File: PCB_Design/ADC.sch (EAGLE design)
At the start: 15 parts, among them J1-0 AD_CH0- GND option, J1-1 AD_CH1- GND option, J1-2 AD_CH2- GND option, J1-3 AD_CH3- GND option, J1-4 AD_CH4- GND option, J1-5 AD_CH5- GND option, J2 Input Screw-terminal Connector, J3 PMOD Interface Connector, X1 4MHz

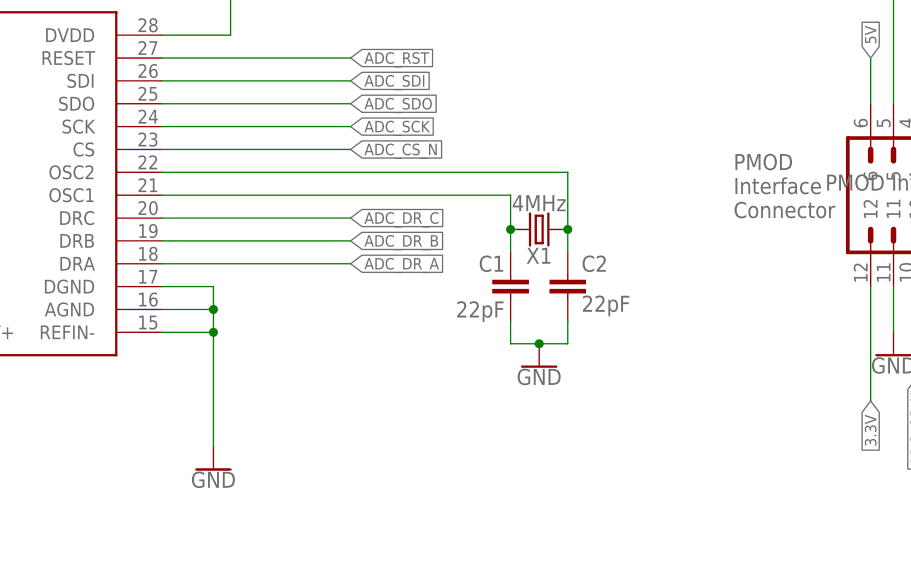
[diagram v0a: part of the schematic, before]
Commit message: Add files via upload
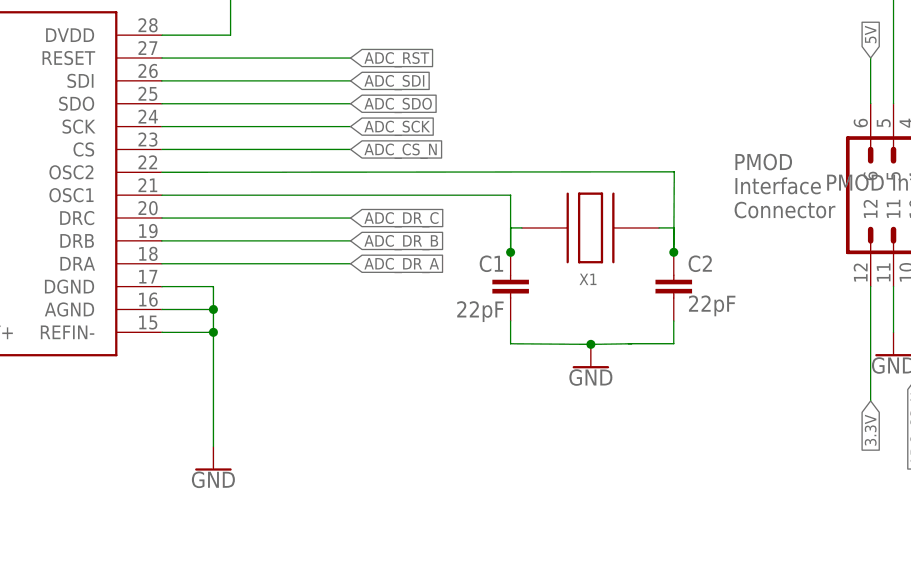
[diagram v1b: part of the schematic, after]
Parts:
- X1: value 4MHz -> 4MHZ; device SparkFun-Clocks:CRYSTALSMD-MC146 -> CalPlug:QUARTZ_3.58M_2PIN
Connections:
- new net N$1: C2.2
- net GND: no longer C2.2
- net OSC_1: now also X1.1; no longer X1.2
- net OSC_2: now also X1.2; no longer X1.1
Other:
- moved on the sheet: C2, X1
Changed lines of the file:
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@@
 <setting verticaltext="up"/>
 </settings>
-<grid distance="0.025" unitdist="inch" unit="inch" style="lines" multiple="1" display="no" altdistance="0.01" altunitdist="inch" altunit="inch"/>
+<grid distance="0.00001" unitdist="inch" unit="inch" style="lines" multiple="1" display="no" altdistance="0.01" altunitdist="inch" altunit="inch"/>
 <layers>
 <layer number="1" name="Top" color="4" fill="1" visible="no" active="no"/>
@@
 <part name="GND9" library="SparkFun-PowerSymbols" deviceset="GND" device=""/>
 <part name="GND11" library="SparkFun-PowerSymbols" deviceset="GND" device=""/>
-<part name="X1" library="SparkFun-Clocks" deviceset="CRYSTAL" device="SMD-MC146" value="4MHz"/>
 <part name="J1-5" library="jumper" library_urn="urn:adsk.eagle:library:252" deviceset="SJ" device="" package3d_urn="urn:adsk.eagle:package:15471/1" value="AD_CH5- GND option"/>
+<part name="X1" library="CalPlug" deviceset="QUARTZ_3.58M_2PIN" device="" value="4MHZ"/>
 </parts>
 <sheets>
@@
 <attribute name="VALUE" x="60.579" y="75.311" size="1.778" layer="96" font="vector"/>
 </instance>
-<instance part="C2" gate="G$1" x="73.025" y="77.47">
-<attribute name="NAME" x="74.549" y="80.391" size="1.778" layer="95" font="vector"/>
-<attribute name="VALUE" x="74.549" y="75.946" size="1.778" layer="96" font="vector"/>
+<instance part="C2" gate="G$1" x="84.80551875" y="77.472540625">
+<attribute name="NAME" x="86.32951875" y="80.393540625" size="1.778" layer="95" font="vector"/>
+<attribute name="VALUE" x="86.32951875" y="75.948540625" size="1.778" layer="96" font="vector"/>
 </instance>
 <instance part="J1-0" gate="1" x="-43.815" y="118.11">
@@
 <attribute name="VALUE" x="-54.61" y="59.436" size="1.778" layer="96" align="top-center"/>
 </instance>
-<instance part="GND9" gate="1" x="69.85" y="69.85">
-<attribute name="VALUE" x="69.85" y="69.596" size="1.778" layer="96" align="top-center"/>
+<instance part="GND9" gate="1" x="75.596240625" y="69.783453125">
+<attribute name="VALUE" x="75.596240625" y="69.529453125" size="1.778" layer="96" align="top-center"/>
 </instance>
 <instance part="GND11" gate="1" x="-54.864" y="92.202">
 <attribute name="VALUE" x="-54.864" y="91.948" size="1.778" layer="96" align="top-center"/>
-</instance>
-<instance part="X1" gate="G$1" x="69.85" y="85.09" rot="R180">
-<attribute name="NAME" x="69.85" y="83.058" size="1.778" layer="95" font="vector" rot="R180" align="bottom-center"/>
-<attribute name="VALUE" x="69.85" y="87.122" size="1.778" layer="96" font="vector" rot="R180" align="top-center"/>
 </instance>
 <instance part="J1-5" gate="1" x="-43.18" y="62.23">
 <attribute name="NAME" x="-41.91" y="60.325" size="1.778" layer="95"/>
 <attribute name="VALUE" x="-50.165" y="58.42" size="1.778" layer="96"/>
+</instance>
+<instance part="X1" gate="G$1" x="75.55738125" y="80.180178125">
+<attribute name="NAME" x="74.28738125" y="78.910178125" size="1.27" layer="95"/>
 </instance>
 </instances>
@@
 <segment>
 <pinref part="C1" gate="G$1" pin="2"/>
-<pinref part="C2" gate="G$1" pin="2"/>
-<wire x1="66.675" y1="72.39" x2="69.85" y2="72.39" width="0.1524" layer="91"/>
-<wire x1="69.85" y1="72.39" x2="73.025" y2="72.39" width="0.1524" layer="91"/>
-<wire x1="73.025" y1="74.93" x2="73.025" y2="72.39" width="0.1524" layer="91"/>
+<wire x1="66.675" y1="72.39" x2="75.596240625" y2="72.323453125" width="0.1524" layer="91"/>
 <wire x1="66.675" y1="72.39" x2="66.675" y2="74.93" width="0.1524" layer="91"/>
 <pinref part="GND9" gate="1" pin="GND"/>
-<junction x="69.85" y="72.39"/>
+<junction x="75.596240625" y="72.323453125"/>
+<wire x1="75.596240625" y1="72.323453125" x2="80.14461875" y2="72.39" width="0.1524" layer="91"/>
 </segment>
 <segment>
@@
 <net name="OSC_1" class="0">
 <segment>
-<wire x1="67.31" y1="85.09" x2="66.675" y2="85.09" width="0.1524" layer="91"/>
 <pinref part="C1" gate="G$1" pin="1"/>
-<wire x1="66.675" y1="82.55" x2="66.675" y2="85.09" width="0.1524" layer="91"/>
 <pinref part="U$1" gate="G$1" pin="OSC1"/>
 <wire x1="27.94" y1="88.9" x2="66.675" y2="88.9" width="0.1524" layer="91"/>
-<wire x1="66.675" y1="88.9" x2="66.675" y2="85.09" width="0.1524" layer="91"/>
-<junction x="66.675" y="85.09"/>
-<pinref part="X1" gate="G$1" pin="2"/>
+<wire x1="66.675" y1="88.9" x2="66.675" y2="82.55" width="0.1524" layer="91"/>
+<pinref part="X1" gate="G$1" pin="1"/>
+<wire x1="67.93738125" y1="85.260178125" x2="66.675" y2="85.260178125" width="0.1524" layer="91"/>
+<wire x1="66.675" y1="85.260178125" x2="66.675" y2="82.55" width="0.1524" layer="91"/>
+<junction x="66.675" y="82.55"/>
 </segment>
 </net>
@@
 <net name="OSC_2" class="0">
 <segment>
-<wire x1="72.39" y1="85.09" x2="73.025" y2="85.09" width="0.1524" layer="91"/>
 <pinref part="C2" gate="G$1" pin="1"/>
-<wire x1="73.025" y1="85.09" x2="73.025" y2="82.55" width="0.1524" layer="91"/>
 <pinref part="U$1" gate="G$1" pin="OSC2"/>
-<wire x1="27.94" y1="91.44" x2="73.025" y2="91.44" width="0.1524" layer="91"/>
-<wire x1="73.025" y1="91.44" x2="73.025" y2="85.09" width="0.1524" layer="91"/>
-<junction x="73.025" y="85.09"/>
-<pinref part="X1" gate="G$1" pin="1"/>
+<wire x1="27.94" y1="91.44" x2="84.858859375" y2="91.4933375" width="0.1524" layer="91"/>
+<wire x1="84.858859375" y1="91.4933375" x2="84.80551875" y2="82.552540625" width="0.1524" layer="91"/>
+<pinref part="X1" gate="G$1" pin="2"/>
+<wire x1="83.17738125" y1="85.260178125" x2="84.80551875" y2="85.260178125" width="0.1524" layer="91"/>
+<wire x1="84.80551875" y1="85.260178125" x2="84.80551875" y2="82.552540625" width="0.1524" layer="91"/>
+<junction x="84.80551875" y="82.552540625"/>
 </segment>
 </net>
@@
 </segment>
 </net>
+<net name="N$1" class="0">
+<segment>
+<pinref part="C2" gate="G$1" pin="2"/>
+<wire x1="79.764940625" y1="72.3956125" x2="84.80551875" y2="72.3956125" width="0.1524" layer="91"/>
+<wire x1="84.80551875" y1="72.3956125" x2="84.80551875" y2="74.932540625" width="0.1524" layer="91"/>
+</segment>
+</net>
